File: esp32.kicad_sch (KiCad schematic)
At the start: 25 parts, among them IC4 TPS22917DBVR, IC5 TPS22917DBVR, IC6 TPS22917DBVR, J19 ESP GPIOs, J6 UART, U4 ESP32-WROOM-32U

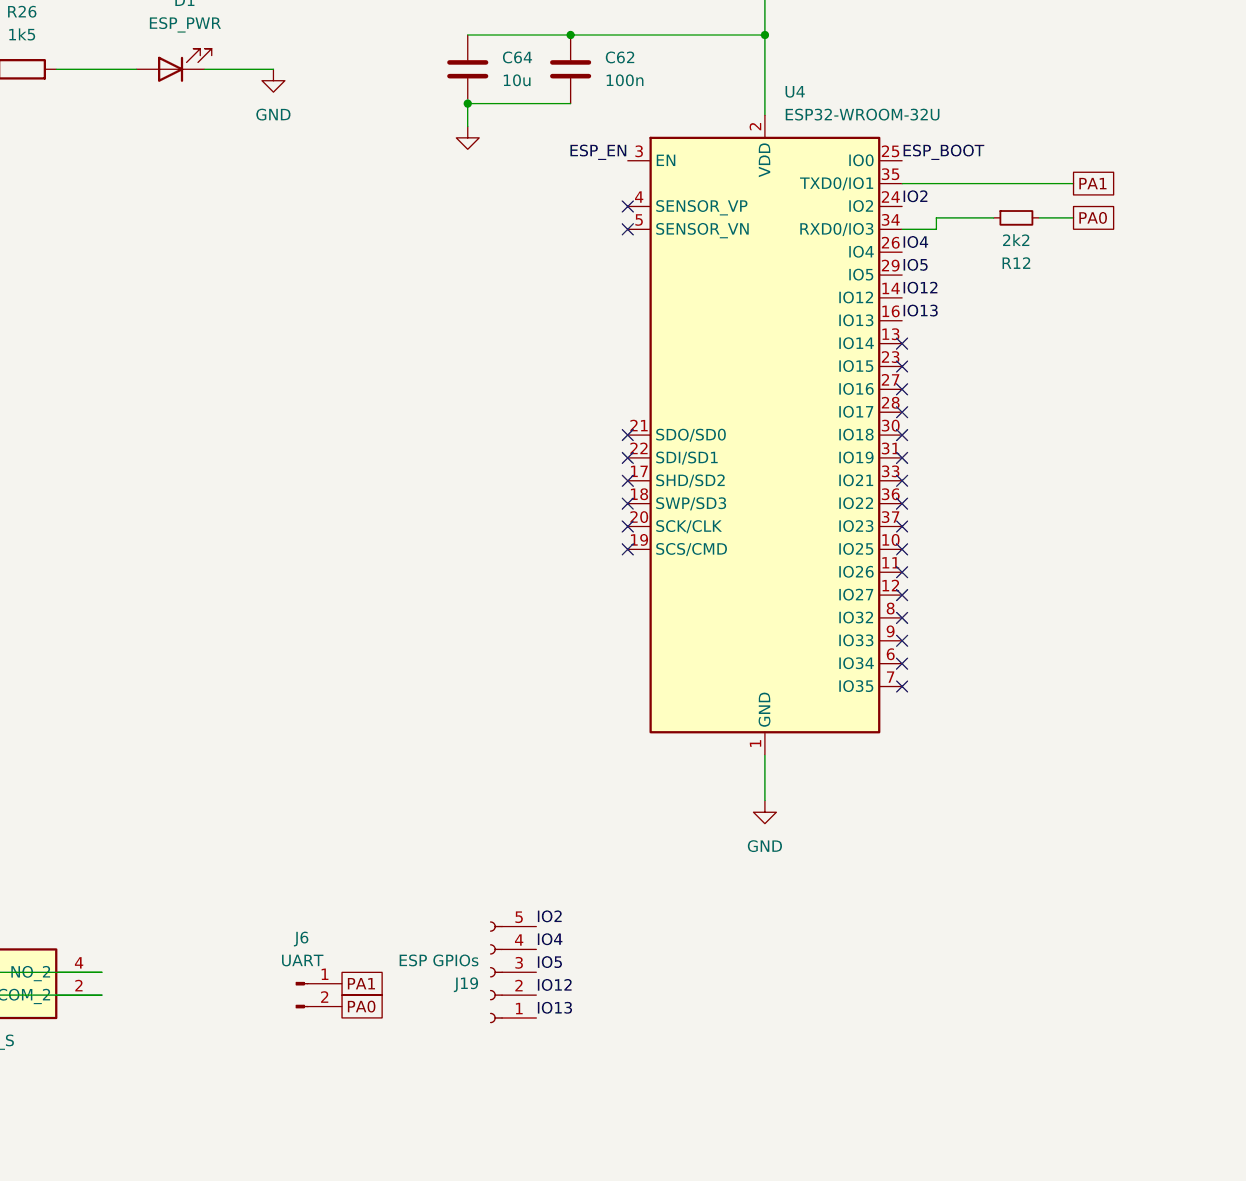
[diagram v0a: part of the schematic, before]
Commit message: Fixed a lot of things
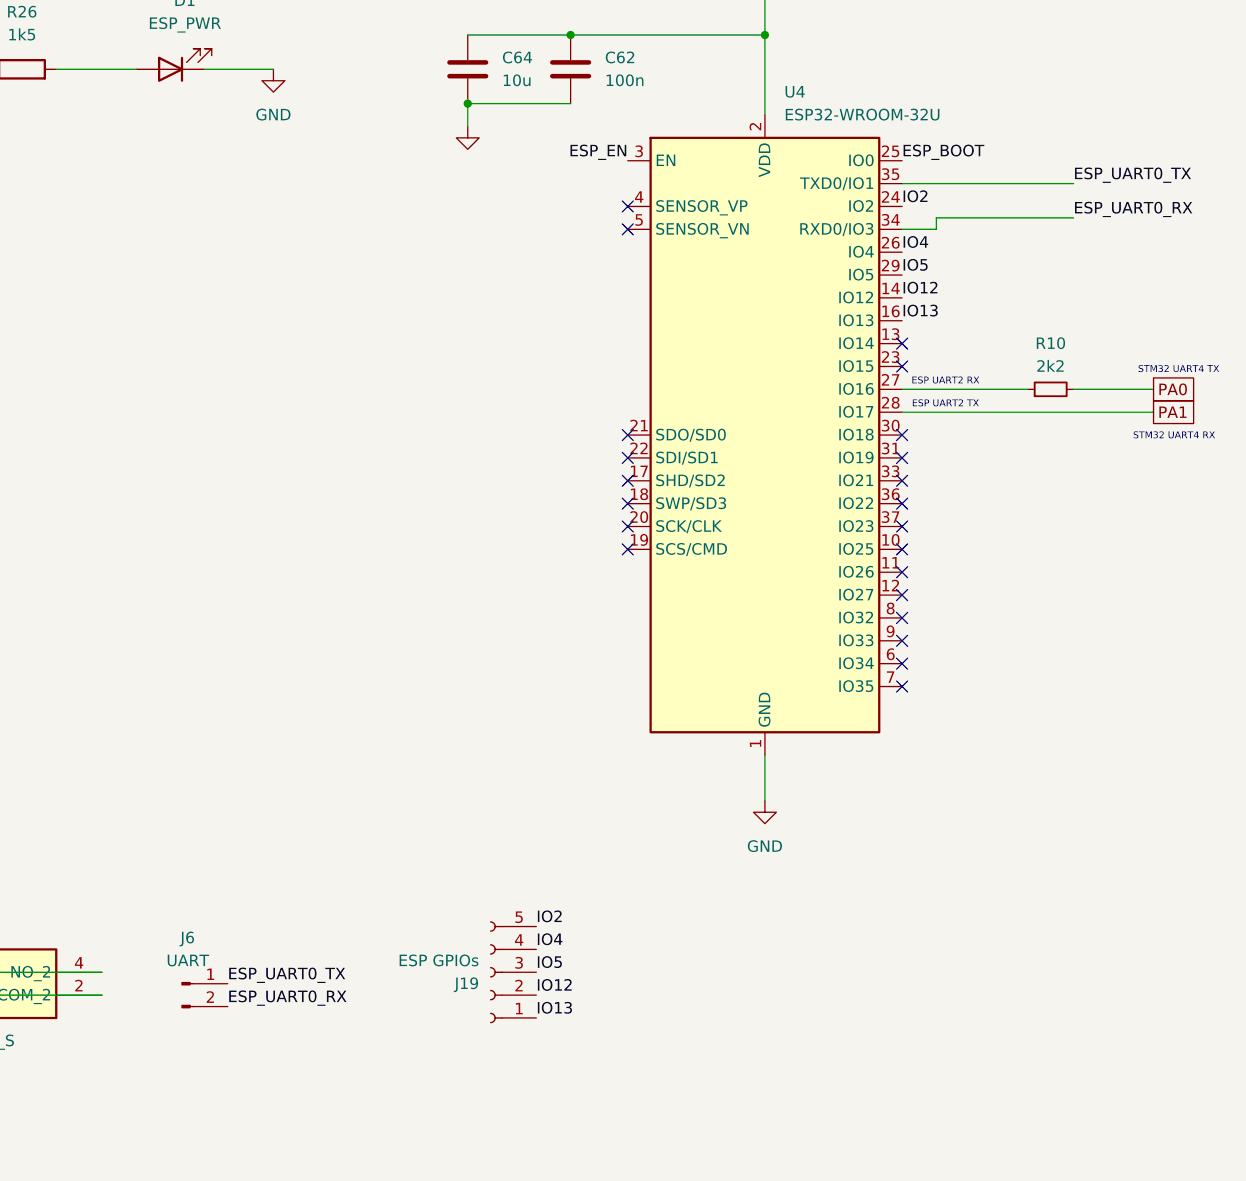
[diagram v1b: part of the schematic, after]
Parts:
- removed R12: 2k2, Resistor_SMD:R_0603_1608Metric_Pad0.98x0.95mm_HandSolder, symbol Device:R_Small
- added R10: 2k2, Resistor_SMD:R_0603_1608Metric_Pad0.98x0.95mm_HandSolder, symbol Device:R_Small
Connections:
- net PA0: now also R10.2; no longer J6.2 (Pin_2)
- net PA1: now also U4.28 (IO17); no longer J6.1 (Pin_1), U4.35 (TXD0/IO1)
- net at U4.27 (IO16): now also R10.1
- net ESP_UART0_RX: now reaches U4.34 (RXD0/IO3)
- net ESP_UART0_RX: now also J6.2 (Pin_2)
- new net ESP_UART0_TX: J6.1 (Pin_1), U4.35 (TXD0/IO1)
- no-connect marks 27 -> 25
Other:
- note added: "ESP UART2 RX"
- note added: "ESP UART2 TX"
- note added: "STM32 UART4 RX"
- note added: "STM32 UART4 TX"
- moved on the sheet: J6
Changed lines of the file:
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@@
 	(generator_version "9.0")
 	(paper "A4")
+	(text "STM32 UART4 TX"
+		(exclude_from_sim no)
+		(at 269.494 72.898 0)
+		(effects
+			(font
+				(size 0.762 0.762)
+			)
+		)
+	)
+	(text "STM32 UART4 RX"
+		(exclude_from_sim no)
+		(at 268.986 80.264 0)
+		(effects
+			(font
+				(size 0.762 0.762)
+			)
+		)
+	)
+	(text "ESP UART2 RX"
+		(exclude_from_sim no)
+		(at 243.586 74.168 0)
+		(effects
+			(font
+				(size 0.762 0.762)
+			)
+		)
+	)
+	(text "ESP UART2 TX"
+		(exclude_from_sim no)
+		(at 243.586 76.708 0)
+		(effects
+			(font
+				(size 0.762 0.762)
+			)
+		)
+	)
 	(junction
 		(at 52.07 147.32)
@@
 	)
 	(no_connect
-		(at 238.76 77.47)
-	)
-	(no_connect
 		(at 238.76 80.01)
 	)
@@
 	)
 	(no_connect
-		(at 238.76 74.93)
-	)
-	(no_connect
 		(at 86.36 107.95)
 	)
@@
 	(wire
 		(pts
+			(xy 238.76 74.93) (xy 252.73 74.93)
+		)
+		(stroke
+			(width 0)
+			(type default)
+		)
+	)
+	(wire
+		(pts
 			(xy 31.75 72.39) (xy 31.75 74.93)
 		)
@@
 	(wire
 		(pts
-			(xy 257.81 55.88) (xy 254 55.88)
-		)
-		(stroke
-			(width 0)
-			(type default)
-		)
-	)
-	(wire
-		(pts
 			(xy 119.38 139.7) (xy 149.86 139.7)
 		)
@@
 	(wire
 		(pts
+			(xy 238.76 77.47) (xy 266.7 77.47)
+		)
+		(stroke
+			(width 0)
+			(type default)
+		)
+	)
+	(wire
+		(pts
 			(xy 58.42 40.64) (xy 31.75 40.64)
 		)
@@
 	(wire
 		(pts
+			(xy 266.7 74.93) (xy 257.81 74.93)
+		)
+		(stroke
+			(width 0)
+			(type default)
+		)
+	)
+	(wire
+		(pts
 			(xy 96.52 139.7) (xy 106.68 139.7)
 		)
@@
 	(wire
 		(pts
-			(xy 248.92 55.88) (xy 242.57 55.88)
+			(xy 242.57 55.88) (xy 257.81 55.88)
 		)
 		(stroke
@@
 		)
 	)
+	(label "ESP_UART0_RX"
+		(at 257.81 55.88 0)
+		(effects
+			(font
+				(size 1.27 1.27)
+			)
+			(justify left bottom)
+		)
+	)
 	(label "ESP_EN"
 		(at 39.37 139.7 180)
@@
 		)
 	)
+	(label "ESP_UART0_TX"
+		(at 257.81 52.07 0)
+		(effects
+			(font
+				(size 1.27 1.27)
+			)
+			(justify left bottom)
+		)
+	)
 	(label "IO4"
 		(at 198.12 137.16 0)
@@
 		)
 	)
+	(label "ESP_UART0_RX"
+		(at 163.83 143.51 0)
+		(effects
+			(font
+				(size 1.27 1.27)
+			)
+			(justify left bottom)
+		)
+	)
 	(label "ESP_ON"
 		(at 88.9 173.99 0)
@@
 		)
 	)
+	(label "ESP_UART0_TX"
+		(at 163.83 140.97 0)
+		(effects
+			(font
+				(size 1.27 1.27)
+			)
+			(justify left bottom)
+		)
+	)
 	(label "NOTE_ON"
 		(at 58.42 107.95 180)
@@
 	(global_label "PA0"
 		(shape passive)
-		(at 176.53 143.51 0)
-		(fields_autoplaced yes)
-		(effects
-			(font
-				(size 1.27 1.27)
-			)
-			(justify left)
-		)
-		(property "Intersheetrefs" "${INTERSHEET_REFS}"
-			(at 181.972 143.51 0)
-			(effects
-				(font
-					(size 1.27 1.27)
-				)
-				(justify left)
-				(hide yes)
-			)
-		)
-	)
-	(global_label "PA0"
-		(shape passive)
-		(at 257.81 55.88 0)
-		(fields_autoplaced yes)
-		(effects
-			(font
-				(size 1.27 1.27)
-			)
-			(justify left)
-		)
-		(property "Intersheetrefs" "${INTERSHEET_REFS}"
-			(at 263.252 55.88 0)
-			(effects
-				(font
-					(size 1.27 1.27)
-				)
-				(justify left)
-				(hide yes)
-			)
-		)
-	)
-	(global_label "PA1"
-		(shape passive)
-		(at 257.81 52.07 0)
+		(at 266.7 74.93 0)
 		(fields_autoplaced yes)
 		(effects
@@
 		)
 		(property "Intersheetrefs" "${INTERSHEET_REFS}"
-			(at 263.252 52.07 0)
+			(at 272.142 74.93 0)
 			(effects
 				(font
@@
 	(global_label "PA1"
 		(shape passive)
-		(at 176.53 140.97 0)
+		(at 266.7 77.47 0)
 		(fields_autoplaced yes)
 		(effects
@@
 		)
 		(property "Intersheetrefs" "${INTERSHEET_REFS}"
-			(at 181.972 140.97 0)
+			(at 272.142 77.47 0)
 			(effects
 				(font
@@
 	)
 	(symbol
-		(lib_id "Device:C")
-		(at 201.93 39.37 0)
+		(lib_id "Device:R_Small")
+		(at 255.27 74.93 90)
 		(unit 1)
 		(exclude_from_sim no)
@@
 		(dnp no)
 		(fields_autoplaced yes)
-		(property "Reference" "C62"
-			(at 205.74 38.0999 0)
+		(property "Reference" "R10"
+			(at 255.27 69.85 90)
 			(effects
 				(font
 					(size 1.27 1.27)
 				)
-				(justify left)
 			)
 		)
-		(property "Value" "100n"
-			(at 205.74 40.6399 0)
+		(property "Value" "2k2"
+			(at 255.27 72.39 90)
 			(effects
 				(font
 					(size 1.27 1.27)
 				)
-				(justify left)
 			)
 		)
-		(property "Footprint" "Capacitor_SMD:C_0603_1608Metric_Pad1.08x0.95mm_HandSolder"
-			(at 202.8952 43.18 0)
+		(property "Footprint" "Resistor_SMD:R_0603_1608Metric_Pad0.98x0.95mm_HandSolder"
+			(at 255.27 74.93 0)
 			(effects
 				(font
@@
 		)
 		(property "Datasheet" "~"
-			(at 201.93 39.37 0)
+			(at 255.27 74.93 0)
 			(effects
 				(font
@@
 			)
 		)
-		(property "Description" "Unpolarized capacitor"
-			(at 201.93 39.37 0)
+		(property "Description" "Resistor, small symbol"
+			(at 255.27 74.93 0)
 			(effects
 				(font
@@
 			)
 		)
-		(pin "2"
-		)
 		(pin "1"
 		)
+		(pin "2"
+		)
 		(instances
 			(project ""
 				(path "/32c2c747-0685-4927-b759-a1d2bc91875e/a402a0ce-c9ea-466a-871f-9107282f1be8"
-					(reference "C62")
+					(reference "R10")
 					(unit 1)
 				)
@@
 	)
 	(symbol
-		(lib_id "Device:R_Small")
-		(at 251.46 55.88 90)
-		(mirror x)
+		(lib_id "Device:C")
+		(at 201.93 39.37 0)
 		(unit 1)
 		(exclude_from_sim no)
@@
 		(on_board yes)
 		(dnp no)
-		(property "Reference" "R12"
-			(at 251.46 60.96 90)
+		(fields_autoplaced yes)
+		(property "Reference" "C62"
+			(at 205.74 38.0999 0)
 			(effects
 				(font
 					(size 1.27 1.27)
 				)
+				(justify left)
 			)
 		)
-		(property "Value" "2k2"
-			(at 251.46 58.42 90)
+		(property "Value" "100n"
+			(at 205.74 40.6399 0)
 			(effects
 				(font
 					(size 1.27 1.27)
 				)
+				(justify left)
 			)
 		)
-		(property "Footprint" "Resistor_SMD:R_0603_1608Metric_Pad0.98x0.95mm_HandSolder"
-			(at 251.46 55.88 0)
+		(property "Footprint" "Capacitor_SMD:C_0603_1608Metric_Pad1.08x0.95mm_HandSolder"
+			(at 202.8952 43.18 0)
 			(effects
 				(font
@@
 		)
 		(property "Datasheet" "~"
-			(at 251.46 55.88 0)
+			(at 201.93 39.37 0)
 			(effects
 				(font
@@
 			)
 		)
-		(property "Description" "Resistor, small symbol"
-			(at 251.46 55.88 0)
+		(property "Description" "Unpolarized capacitor"
+			(at 201.93 39.37 0)
 			(effects
 				(font
@@
 		)
 		(instances
-			(project "telemetry-rusolar-rework"
+			(project ""
 				(path "/32c2c747-0685-4927-b759-a1d2bc91875e/a402a0ce-c9ea-466a-871f-9107282f1be8"
-					(reference "R12")
+					(reference "C62")
 					(unit 1)
 				)
@@
 	(symbol
 		(lib_id "Connector:Conn_01x02_Pin")
-		(at 171.45 140.97 0)
+		(at 158.75 140.97 0)
 		(unit 1)
 		(exclude_from_sim no)
@@
 		(fields_autoplaced yes)
 		(property "Reference" "J6"
-			(at 172.085 135.89 0)
+			(at 159.385 135.89 0)
 			(effects
 				(font
@@
 		)
 		(property "Value" "UART"
-			(at 172.085 138.43 0)
+			(at 159.385 138.43 0)
 			(effects
 				(font
@@
 		)
 		(property "Footprint" "Connector_PinHeader_2.00mm:PinHeader_1x02_P2.00mm_Vertical"
-			(at 171.45 140.97 0)
+			(at 158.75 140.97 0)
 			(effects
 				(font
@@
 		)
 		(property "Datasheet" "~"
-			(at 171.45 140.97 0)
+			(at 158.75 140.97 0)
 			(effects
 				(font
@@
 		)
 		(property "Description" "Generic connector, single row, 01x02, script generated"
-			(at 171.45 140.97 0)
+			(at 158.75 140.97 0)
 			(effects
 				(font
